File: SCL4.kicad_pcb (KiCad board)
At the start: 2 copper layers, 150.5 x 233.3 mm, 38 parts, among them J1 spare1, J2 spare2, J3 Siemens_A1010-A263, J4 SP1, J5 SP2, J6 Conn_01x08, J7 5V out, U1 MC3487DX, U2 MC3487DX, U3 TRAM Size 2, U4 MC10H125 (20PLCC), U5 MC10H124 (20PLCC)

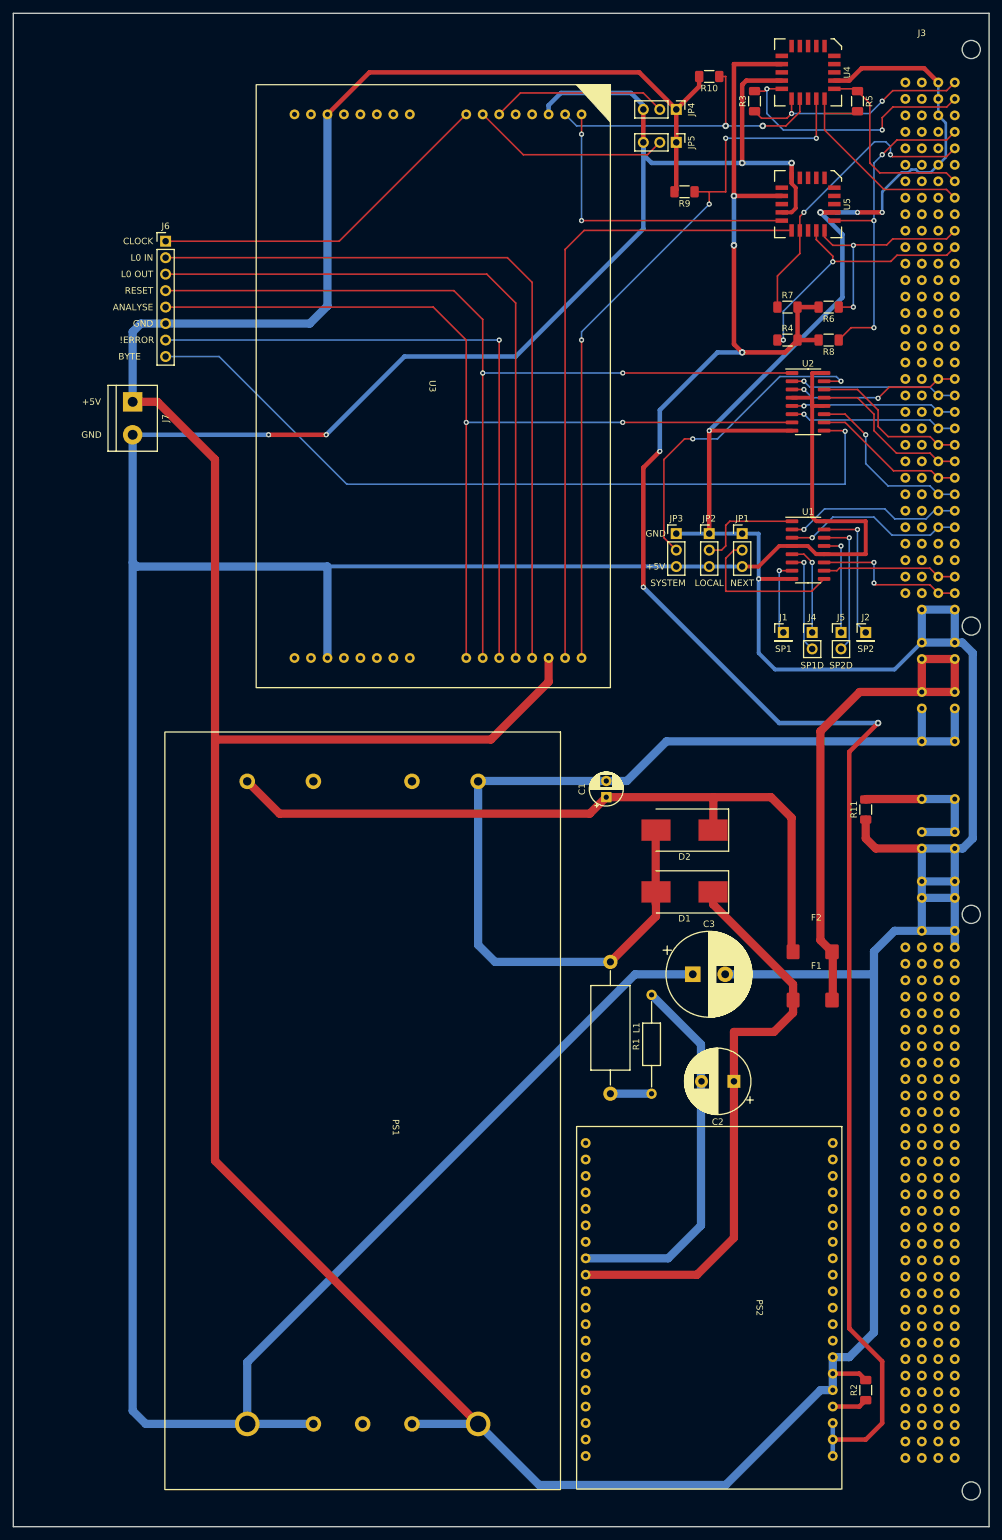
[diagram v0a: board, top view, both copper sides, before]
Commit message: polish
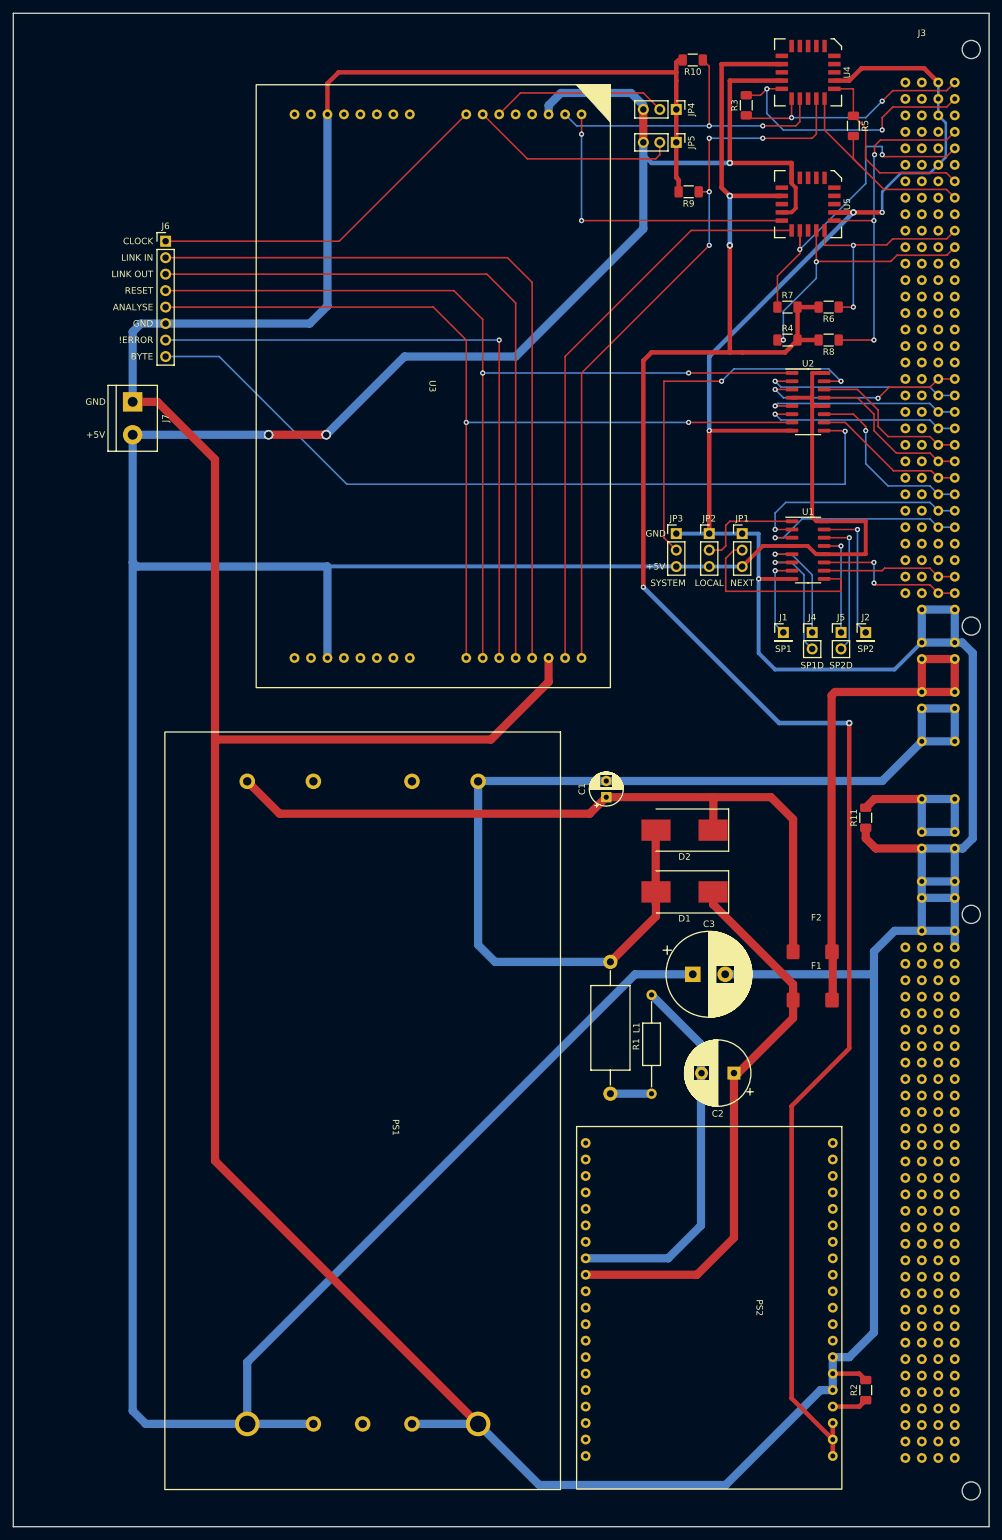
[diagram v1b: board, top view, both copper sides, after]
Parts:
- moved R5 3.86 mm to (283.8, 33.7)
- moved R10 3.59 mm to (259.1, 23.5)
- moved R3 1.42 mm to (267.3, 30.5)
- moved R11 1.27 mm to (285.8, 140.3)
- moved C2 1.27 mm to (265.4, 179.7)
- moved R9 0.63 mm to (258.4, 43.8)
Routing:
- net /TL3out: track 99.1 -> 89.5 mm
- net Net-(JP3-Pad2): track 50.3 -> 58.3 mm
- net /LOCAL: track 27.6 -> 34.1 mm
- net Net-(JP1-Pad2): track 24.1 -> 30.4 mm
- net //L2OUT: track 46.3 -> 51.9 mm
- net /Static: track 23.9 -> 29.5 mm
- net //ANALYSE: track 25.6 -> 31.0 mm
- net /ANALYSE: track 26.0 -> 31.2 mm
- net /RESET: track 26.0 -> 31.2 mm
- net //RESET: track 26.9 -> 32.1 mm
- net -48V: track 156.7 -> 161.8 mm
- net Net-(J4-Pad1): track 14.4 -> 18.5 mm
- net Net-(J4-Pad2): track 15.7 -> 19.8 mm
- net //LOCAL: track 28.1 -> 32.0 mm
- net Net-(C2-Pad1): track 91.1 -> 87.8 mm
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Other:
- board text added: "LINK IN"
- board text added: "LINK OUT"
- board text removed: "L0 IN"
- board text removed: "L0 OUT"
